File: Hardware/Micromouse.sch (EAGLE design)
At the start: 12 parts, among them IC1 LM324N

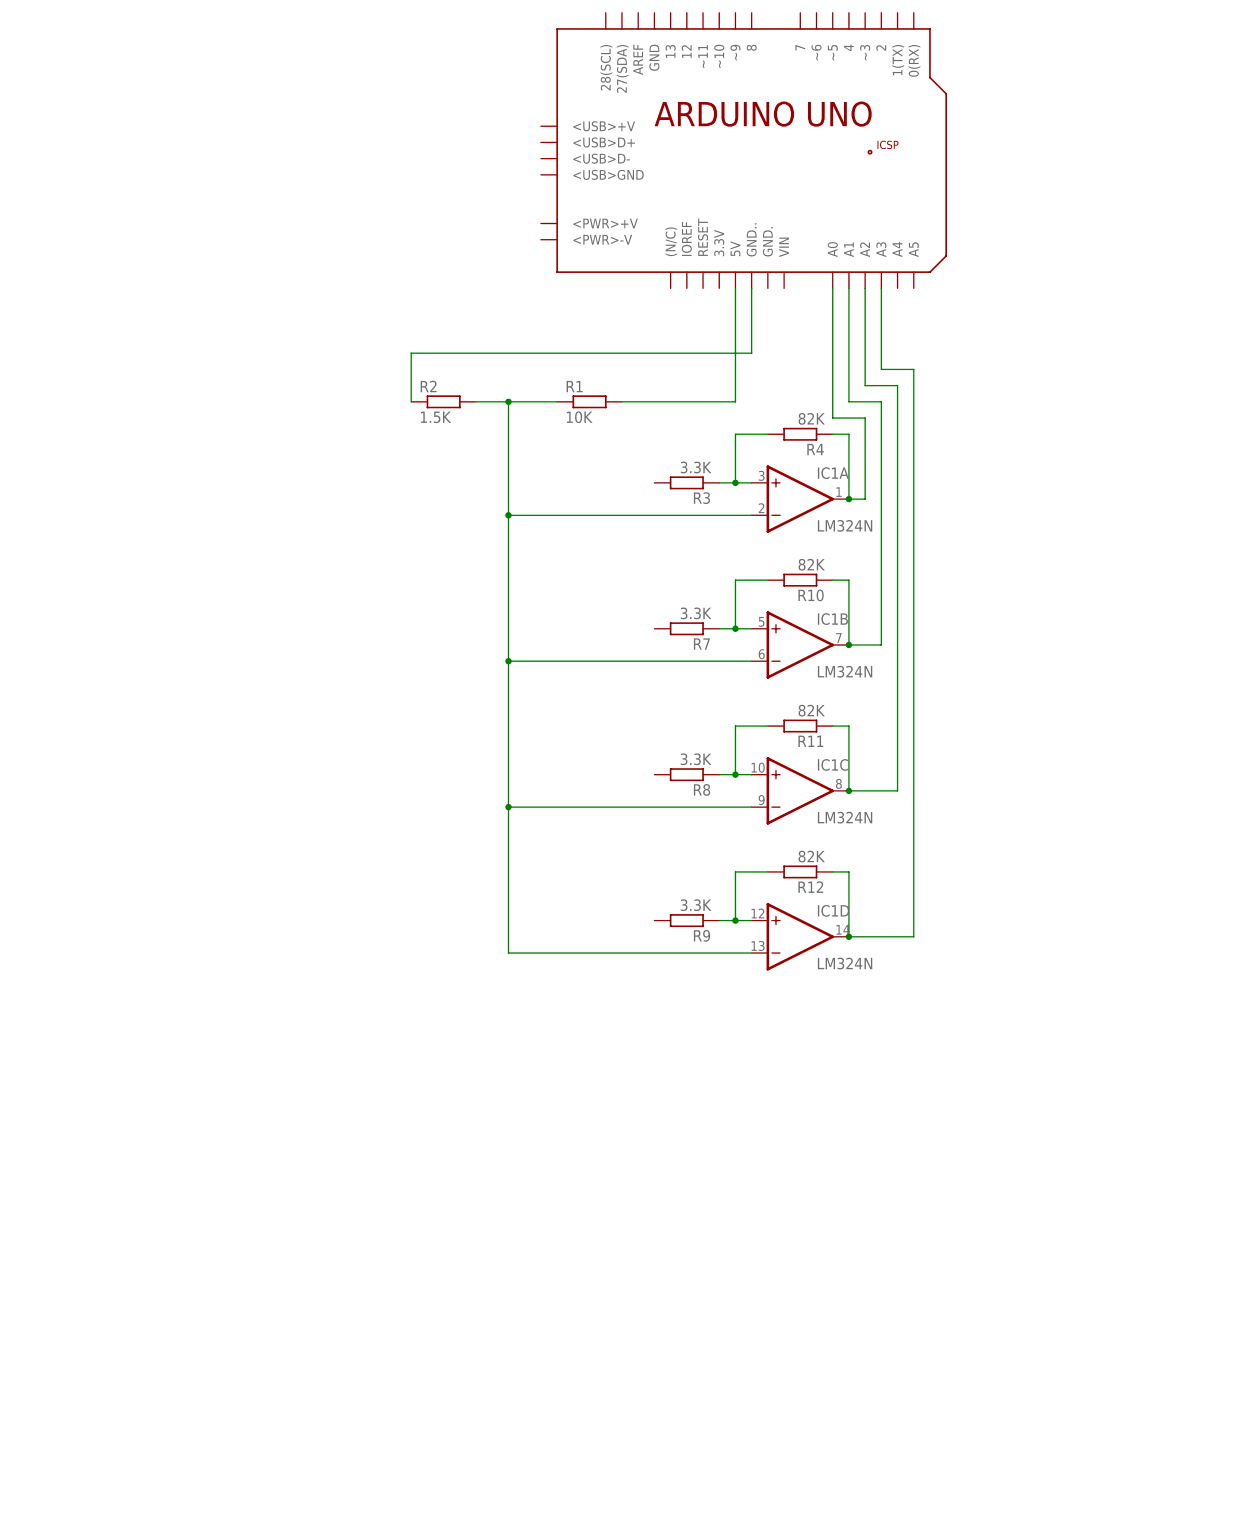
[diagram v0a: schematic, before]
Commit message: Updated hardware + schematic complete + Board almost done but looks a bit terrible
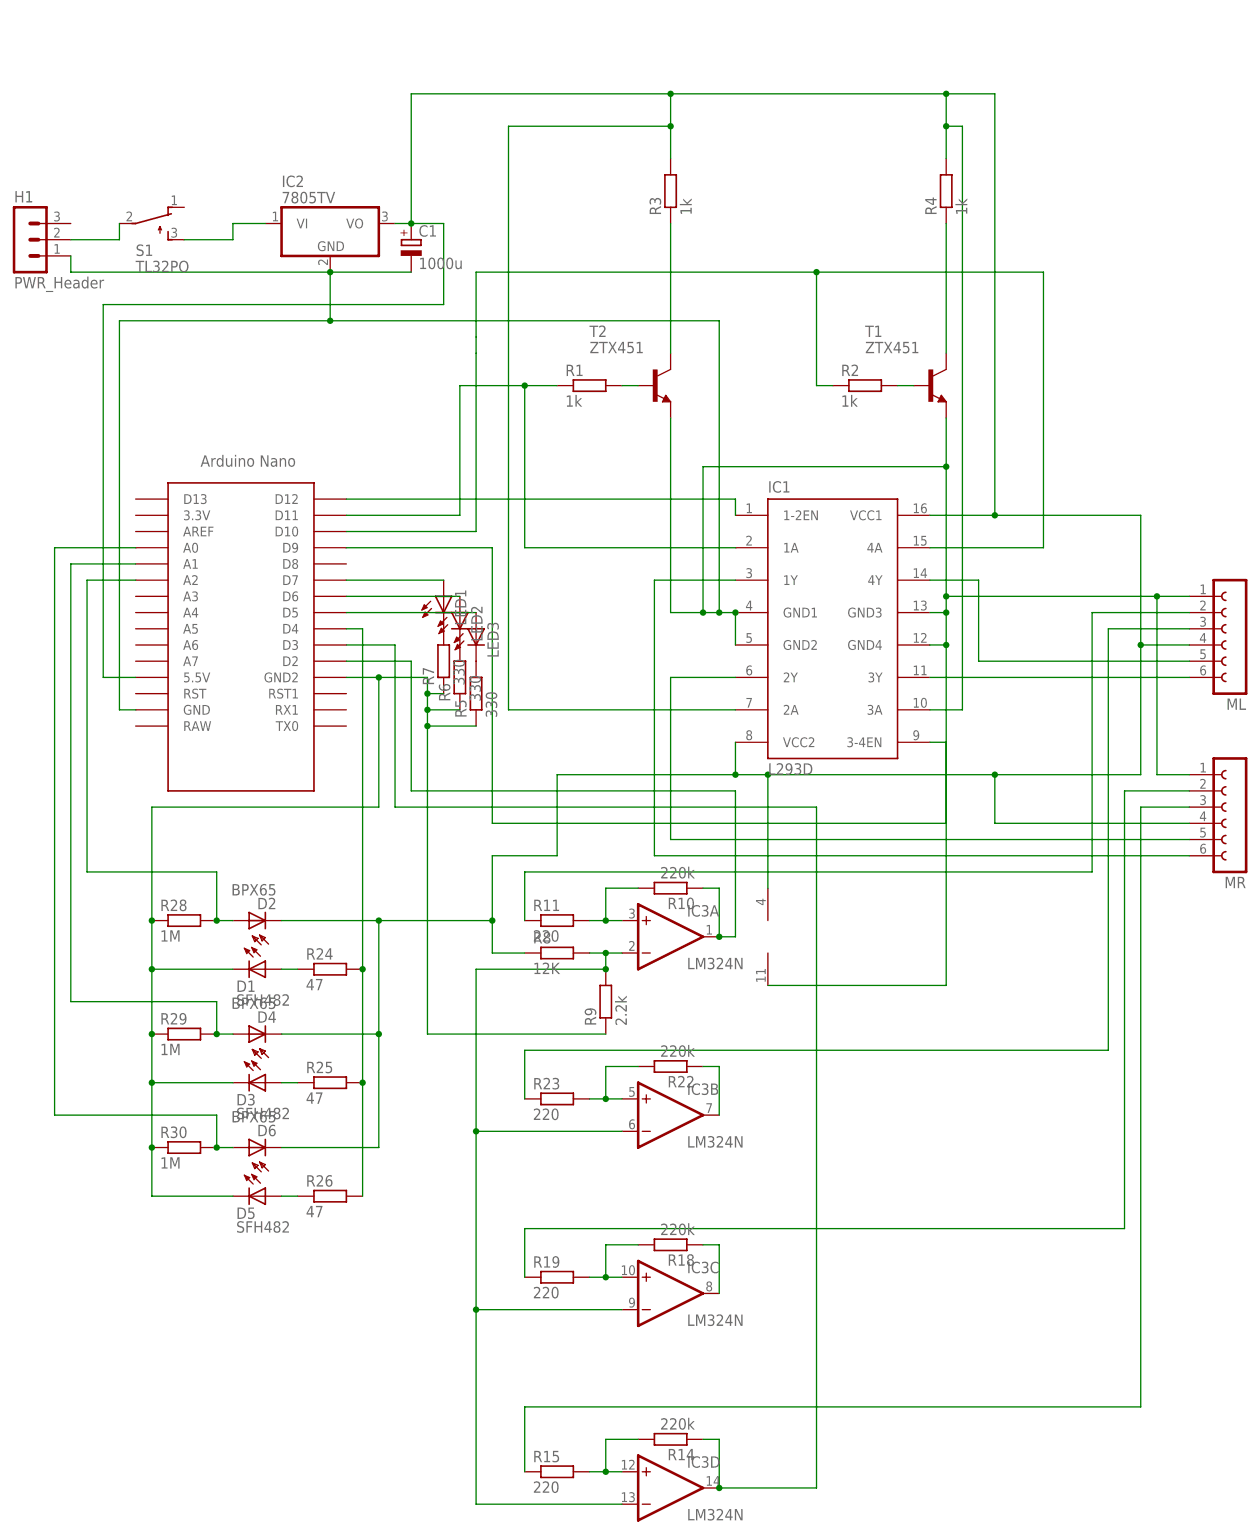
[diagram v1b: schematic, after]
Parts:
- removed PCB1: ARDUINO_UNO_EXT, E14_Arduino_revC:ARDUINO_UNO_EXT
- removed R12: 82K, resistor:R-EU_0309/10
- added C1: 1000u, resistor:CPOL-EUE3.5-10
- added D1, D3, D5: SFH482, led:SFH482
- added D2, D4, D6: BPX65, opto-trans-siemens:BPX65
- added H1: PWR_Header, con-lstb:MA03-1
- added IC2: 7805TV, linear:7805TV
- added IC3: LM324N, linear:LM324N
- added LED1, LED2, LED3: (no value), eagle-ltspice:LED_ELD260
- added ML, MR: (no value), con-lsta:FE06-1
- added R14, R18, R22: 220k, eagle-ltspice:R0204/7
- added R15, R19, R23: 220, eagle-ltspice:R0204/7
- added R24, R25, R26: 47, eagle-ltspice:R0204/7
- added R28, R29, R30: 1M, eagle-ltspice:R0204/7
- added R5, R6: 330, eagle-ltspice:R0204/7
- added S1: TL32PO, switch:TL32PO
- added T1, T2: ZTX451, transistor:BC238
- added U$1: NANO, Arduino-clone:NANO
- IC1: value LM324N -> L293D; device linear:LM324N -> st-microelectronics:L293D
- R1: value 10K -> 1k; device resistor:R-EU_0309/10 -> eagle-ltspice:R0204/7
- R10: value 82K -> 220k; device resistor:R-EU_0309/10 -> eagle-ltspice:R0204/7
- R11: value 82K -> 220; device resistor:R-EU_0309/10 -> eagle-ltspice:R0204/7
- R2: value 1.5K -> 1k; device resistor:R-EU_0309/10 -> eagle-ltspice:R0204/7
- R3: value 3.3K -> 1k; device resistor:R-EU_0309/10 -> eagle-ltspice:R0204/7
- R4: value 82K -> 1k; device resistor:R-EU_0309/10 -> eagle-ltspice:R0204/7
- R7: value 3.3K -> 330; device resistor:R-EU_0309/10 -> eagle-ltspice:R0204/7
- R8: value 3.3K -> 12K; device resistor:R-EU_0309/10 -> eagle-ltspice:R0204/7
- R9: value 3.3K -> 2.2k; device resistor:R-EU_0309/10 -> eagle-ltspice:R0204/7
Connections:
- new net 5V: C1.+, D2.C, D4.C, D6.C, IC1.3A, IC1.VCC1, IC1.VCC2, IC2.VO, IC3P.V+, ML.4, MR.4, R3.2, R4.2, R8.1, U$1.5.5V
- new net GND: C1.-, D1.C, D3.C, D5.C, H1.1, IC1.GND1, IC1.GND2, IC1.GND3, IC1.GND4, IC2.GND, IC3P.V-, ML.1, MR.1, R28.1, R29.1, R30.1, R5.1, R6.1, R7.1, R9.1, T1.E, T2.E, U$1.GND, U$1.GND2
- new net N$12: R4.1, T1.C
- new net N$13: IC3B.OUT, R22.1
- new net N$15: LED3.C, R5.2
- new net N$16: IC1.3-4EN, U$1.D9
- new net N$19: LED2.C, R6.2
- new net N$20: LED1.C, R7.2
- new net N$22: IC3A.OUT, R10.1, U$1.D2
- new net N$23: IC3A.+IN, R10.2, R11.2
- new net N$24: LED1.A, U$1.D7
- new net N$25: LED2.A, U$1.D6
- new net N$26: LED3.A, U$1.D5
- new net N$27: IC3A.-IN, IC3B.-IN, IC3C.-IN, IC3D.-IN, R8.2, R9.2
- new net N$28: IC3C.OUT, R18.1
- new net N$29: ML.2, R11.1
- new net N$30: ML.3, R23.1
- new net N$31: IC3D.OUT, R14.1, U$1.D3
- new net N$32: IC3D.+IN, R14.2, R15.2
- new net N$34: MR.2, R19.1
- new net N$35: MR.3, R15.1
- new net N$36: R24.2, R25.2, R26.2, U$1.D4
- new net N$37: IC3C.+IN, R18.2, R19.2
- new net N$39: D4.A, R29.2, U$1.A1
- new net N$40: D5.A, R26.1
- new net N$42: IC3B.+IN, R22.2, R23.2
- new net N$44: D3.A, R25.1
- new net N$45: D1.A, R24.1
- new net N$46: D2.A, R28.2, U$1.A2
- new net N$48: D6.A, R30.2, U$1.A0
- new net VI: IC2.VI, S1.S
- net N$1: now also IC1.3Y, ML.6; no longer PCB1.5V, R1.2
- net N$10: now also IC1.1-2EN, U$1.D12; no longer IC1B.OUT, PCB1.A1, R10.1
- net N$11: now also R3.1, T2.C; no longer IC1B.+IN, R10.2, R7.1
- net N$2: now also IC1.4Y, ML.5; no longer IC1A.-IN, IC1B.-IN, IC1C.-IN, IC1D.-IN, R1.1, R2.2
- net N$3: now also IC1.1Y, MR.6; no longer PCB1.GND.., R2.1
- net N$4: now also IC1.2Y, MR.5; no longer IC1A.+IN, R3.1, R4.2
- net N$5: now also R1.2, T2.B; no longer IC1A.OUT, PCB1.A0, R4.1
- net N$6: now also R2.2, T1.B; no longer IC1D.OUT, PCB1.A3, R12.1
- net N$7: now also IC1.4A, R2.1, U$1.D10; no longer IC1D.+IN, R12.2, R9.1
- net N$8: now also IC1.1A, R1.1, U$1.D11; no longer IC1C.+IN, R11.2, R8.1
- net N$9: now also H1.2, S1.P; no longer IC1C.OUT, PCB1.A2, R11.1
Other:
- moved on the sheet: R1, R10, R11, R2, R3, R4, R7, R8, R9
